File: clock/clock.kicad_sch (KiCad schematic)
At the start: 43 parts, among them J1 Conn_01x06, J2 Power_inlet_vertical, J3 Conn_02x03_Odd_Even, J4 Conn_01x03, J5 Conn_01x03, SW1 Omron_B3F_SPST, SW2 Omron_B3F_SPST, SW3 Omron_B3F_SPST, SW4 Omron_B3F_SPST, U1 ATmega328-PU, U2 L7805, U3 MAX7219, U4 DS1307_DIP-8, Y1 Crystal_16MHz, Y2 Crystal_32768Hz

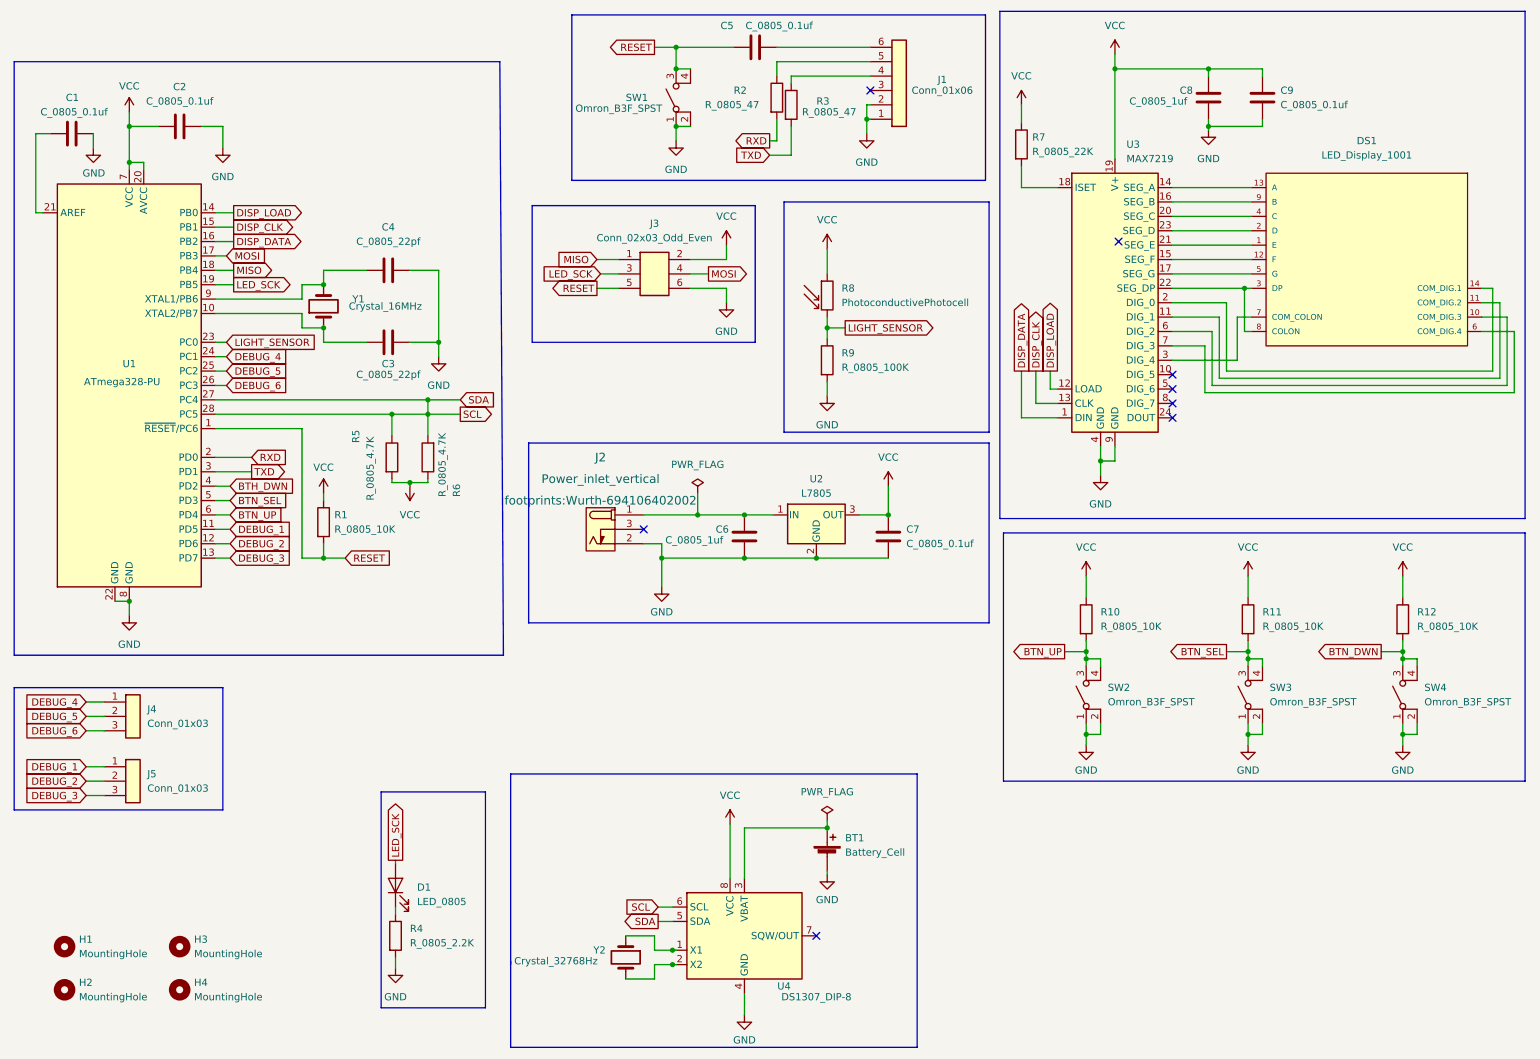
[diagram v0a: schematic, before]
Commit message: did a copper pour
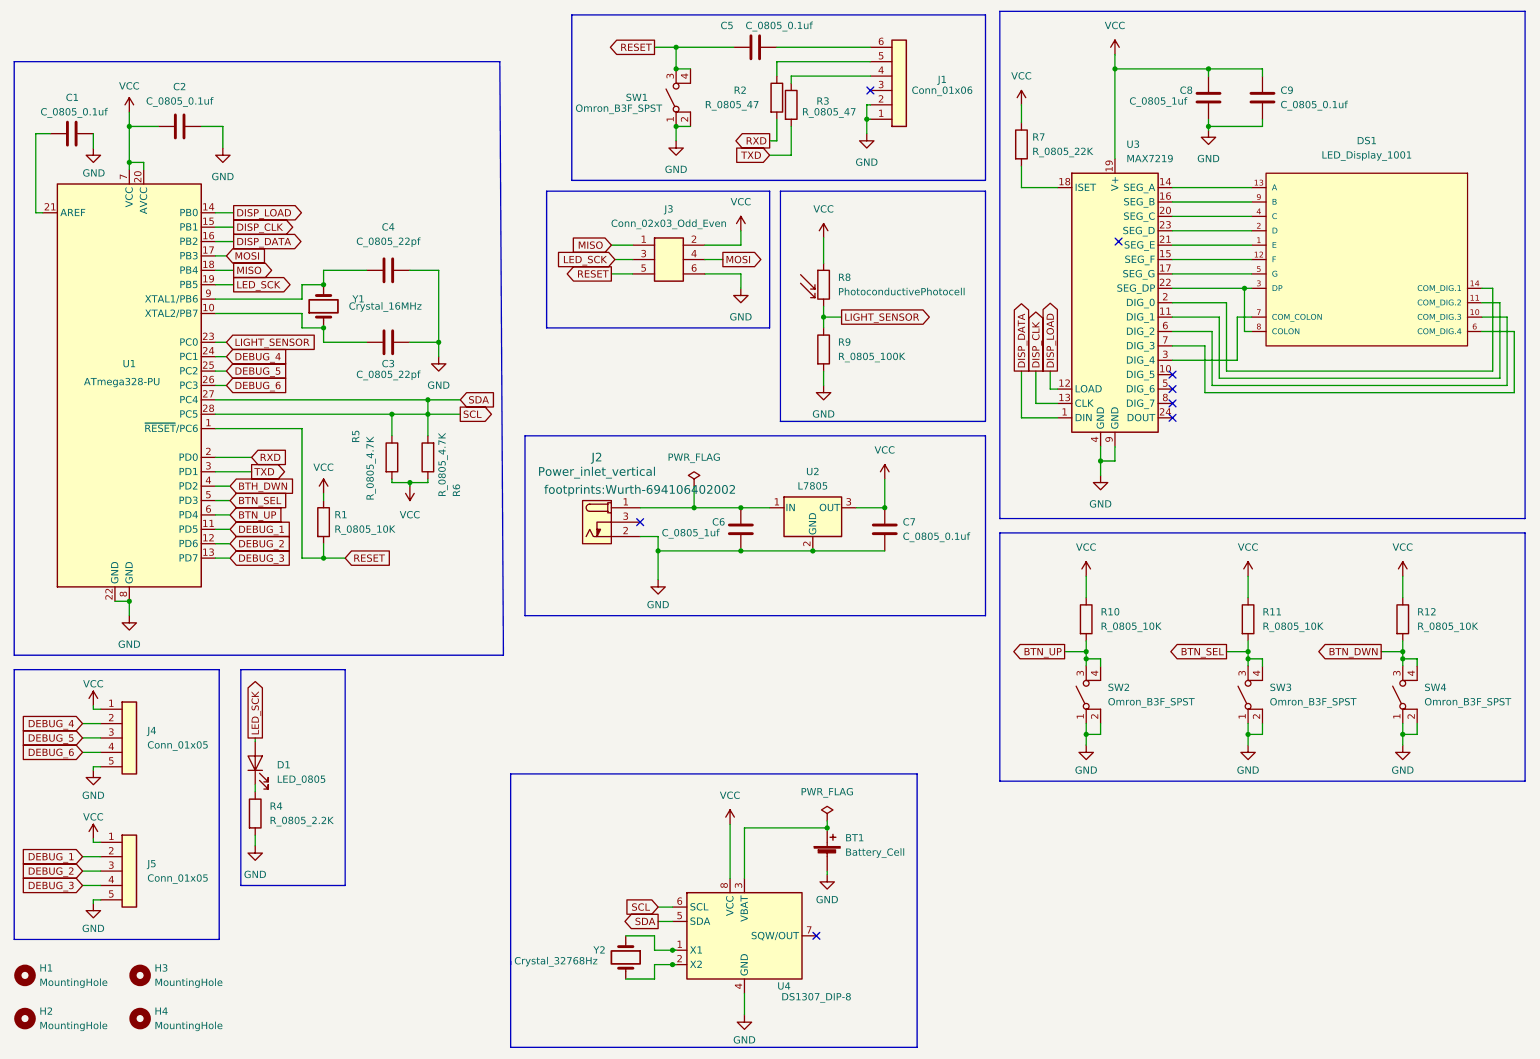
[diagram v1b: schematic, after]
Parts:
- removed J4, J5: Conn_01x03, footprints:PinHeader_1x03_P2.54mm_Vertical, symbol HPS:Conn_01x03
- added J4, J5: Conn_01x05, footprints:PinHeader_1x05_P2.54mm_Vertical, symbol HPS:Conn_01x05
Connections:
- net DEBUG_1: now also J5.2 (Pin_2)
- net DEBUG_2: now also J5.3 (Pin_3)
- net DEBUG_3: now also J5.4 (Pin_4)
- net DEBUG_4: now also J4.2 (Pin_2)
- net DEBUG_5: now also J4.3 (Pin_3)
- net DEBUG_6: now also J4.4 (Pin_4)
- net GND: now also J4.5 (Pin_5), J5.5 (Pin_5)
- net VCC: now also J4.1 (Pin_1), J5.1 (Pin_1)
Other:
- moved on the sheet: C6, C7, D1, H1, H2, H3, H4, J2, J3, R4, R8, R9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
